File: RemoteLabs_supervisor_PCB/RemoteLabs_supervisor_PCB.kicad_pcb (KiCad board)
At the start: 4 copper layers, 180.3 x 99.1 mm, 200 parts, among them J1 Super_Prog_Header, J10 ShiftReg_Header, J11 SPI Student, J12 MCU_Header, J13 USB_B_Mini, J14 ShiftReg_Header, J15 SPI Supervisor, J16 MotorController_PWR_IP, J17 MotorController, J18 DC Motor Output, J19 Stepper Motor Output, J2 WS2821B Header, J20 Servo_A, J21 Servo_B, J22 Thermocouple A, J23 limit_switch_A, J24 limit_switch_B, J25 Optical Encoder, J26 Student_Prog_Header, J27 Analog Buffer, J28 student_PA03, J29 3V3 PWR SRC, J3 XT60_60A_male, J30 12V_DC, J31 5V_DC_RPI, J32 GND_BUS, J33 12V_BUS, J34 5V_P_BUS, J35 5V_D_BUS, J36 3V3_BUS, J4 Strip Lighting, J5 USB_A_Stacked, J6 5V_DC_LED, J7 USB_B_Mini, J8 MCU_Header, J9 Spare Student GPIOs, Q1 IRF5305_PBF, SW1 Stepper_Mode, SW2 Student Reset, SW3 Supervisor Reset, U1 R-78C5.0-1.0, U10 4081, U11 4081, U12 4081, U13 74HC86, U14 74HC86, U15 NCS20074D, U16 NCS20074D, U17 NCS20074D, U18 R-78C5.0-1.0, U19 AD8497, U2 TCYSH14F, U20 74LS07, U21 74LS07, U22 74LS07, U23 TCYSH14F, U3 AMS1117-3.3, U4 ATSAMD21G18A-M, U5 4094, U6 ATSAMD21G18A-M, U7 4094, U8 4069, U9 4081, X1 ASEK-xxxMHz, X2 ASEK-xxxMHz

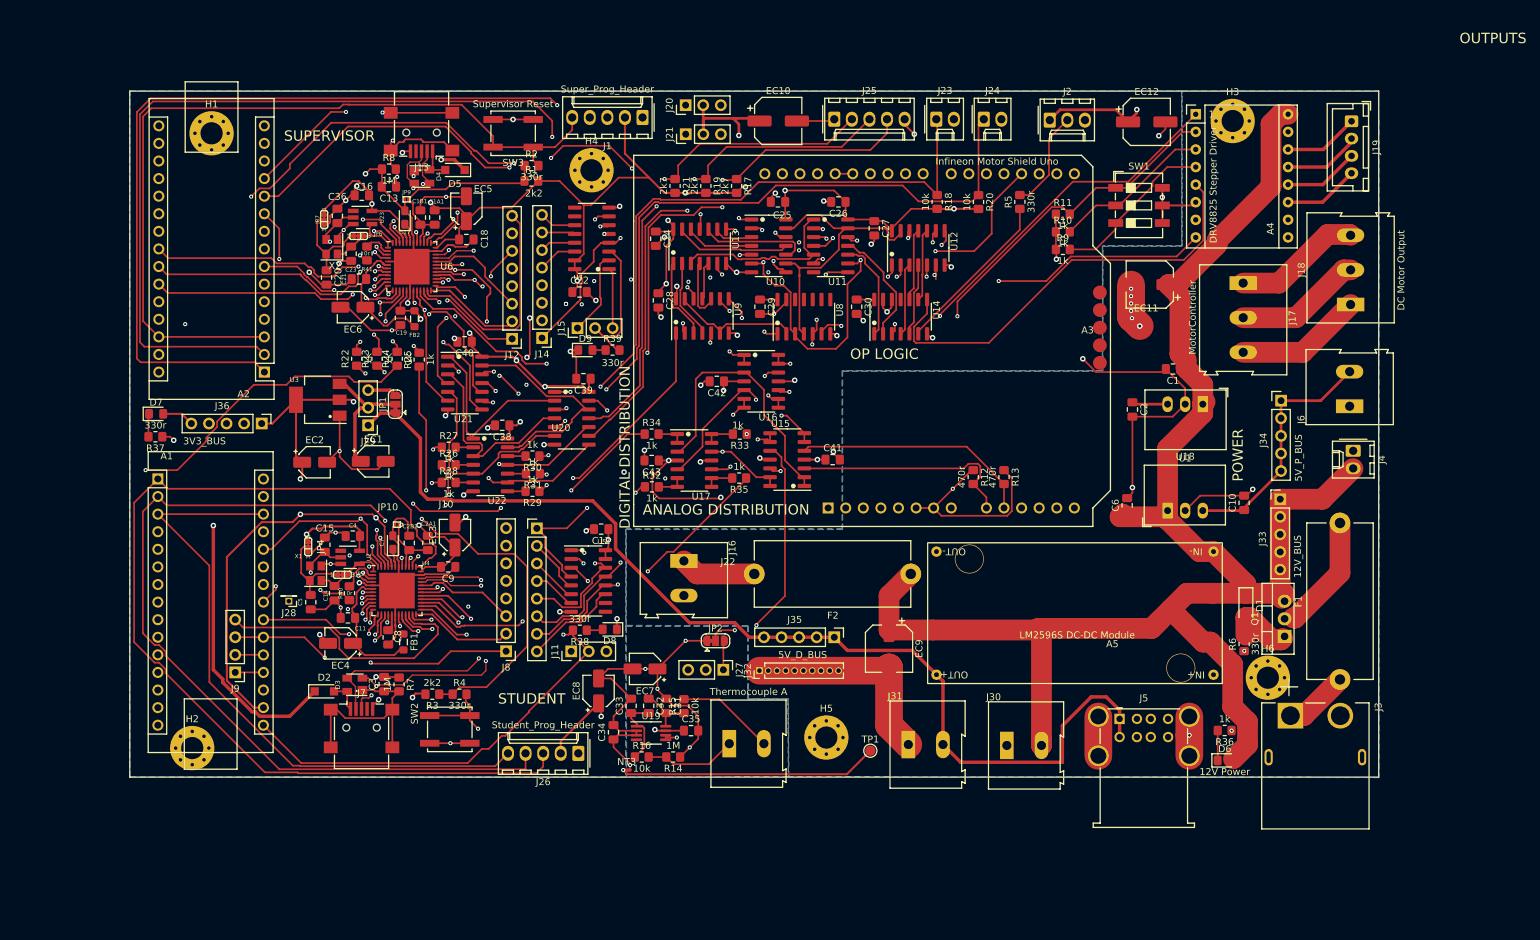
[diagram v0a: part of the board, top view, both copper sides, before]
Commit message: routing board layout 2.0
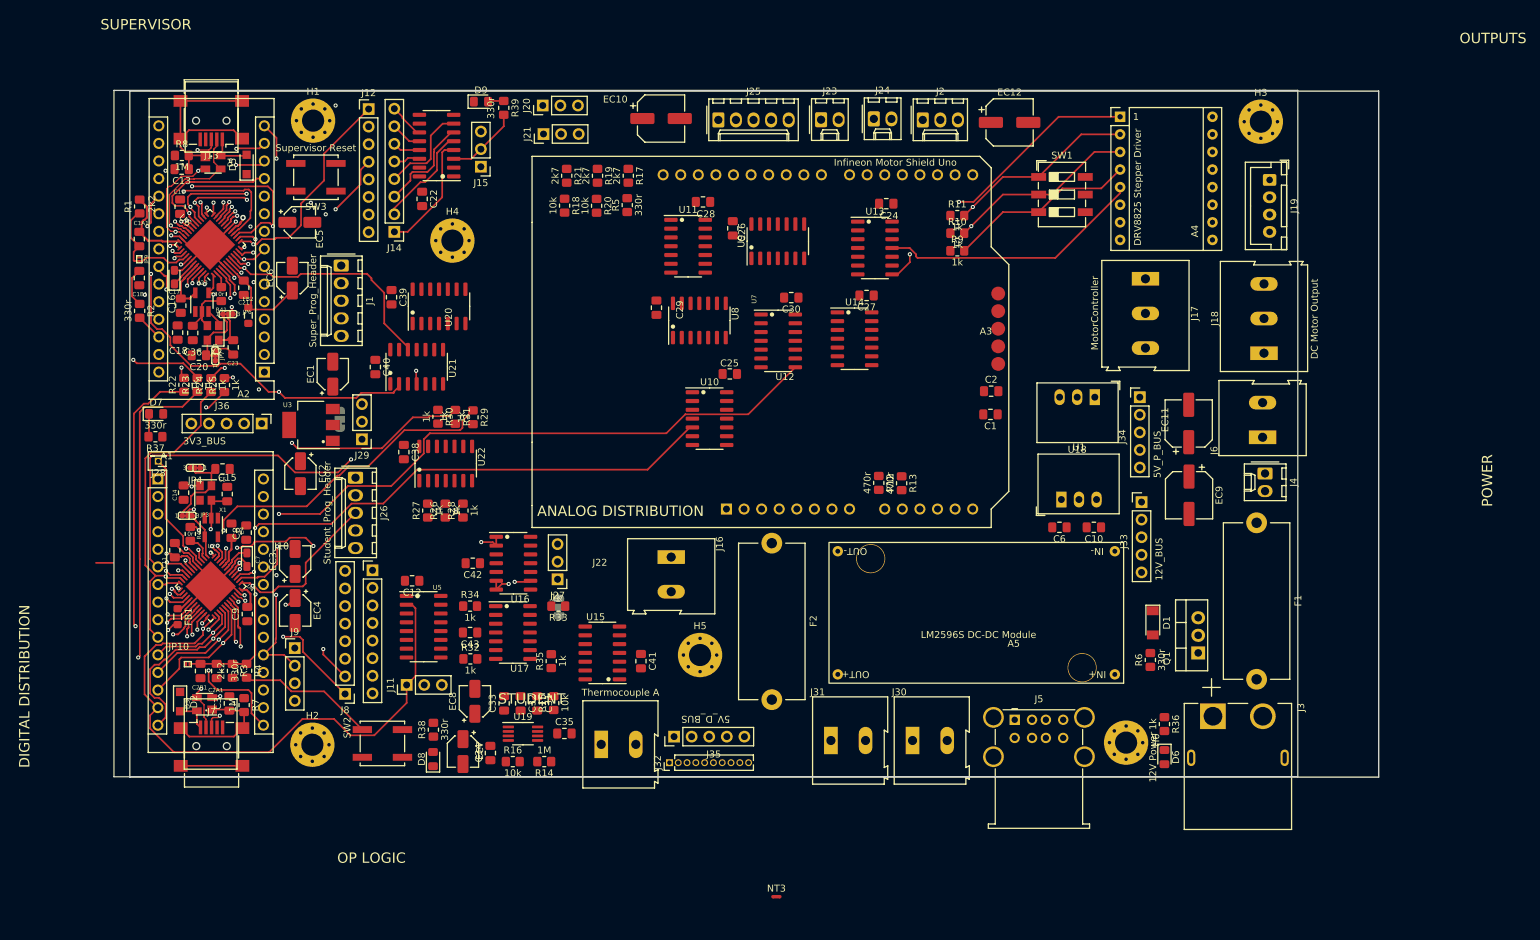
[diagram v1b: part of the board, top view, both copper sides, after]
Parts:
- removed TP1: GND, TestPoint:TestPoint_Pad_D1.5mm
- removed the U12 at (164.7, 45.5)
- added U9: 4081, Package_SO:SOIC-14_3.9x8.7mm_P1.27mm, F.Cu at (144.4, 44.5)
- JP1, JP2: moved to B.Cu
- moved R2 60.4 mm to (52.2, 54.6), turned to -90 degrees
- moved R5 56.7 mm to (122.6, 39.3)
- moved R1 56.7 mm to (52.2, 39.5), turned to 90 degrees
- moved R20 55.1 mm to (118.2, 39.4)
- moved R18 53.8 mm to (113.6, 39.4)
- moved J26 51.2 mm to (83.4, 78.7), turned to -90 degrees
- moved EC9 48.7 mm to (203.8, 81.2)
- moved J1 48.5 mm to (81.3, 48.1), turned to -90 degrees
- moved U16 44.4 mm to (106.2, 91.0)
- moved C42 43.9 mm to (100.3, 91.0)
- moved C18 43.8 mm to (57.7, 57.7), turned to -90 degrees
- moved C1A1 42.8 mm to (52.2, 44.2)
- moved C1B1 41.5 mm to (52.2, 49.9), turned to -90 degrees
- moved C41 40.2 mm to (124.6, 105.2), turned to -90 degrees
- moved JP9 39.6 mm to (52.2, 47.1), turned to -90 degrees
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- renumbered U9 to U12
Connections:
- U10 pad 12: /Output Logic/SUPERVISOR_STEP -> /Output Logic/STUDENT_STEP_RST
- U10 pad 13: Net-(U10-Pad13) -> /Output Logic/MCU_STEP_SELECT
- U10 pad 8: /Output Logic/SUPERVISOR_DIRECTION -> /Output Logic/STUDENT_STEP_EN
- U10 pad 9: Net-(U10-Pad13) -> /Output Logic/MCU_STEP_SELECT
- U11 pad 1: Net-(U11-Pad1) -> /Output Logic/SUPERVISOR_DIRECTION
- U11 pad 12: /Output Logic/SUPERVISOR_STEP_EN -> /Output Logic/SUPERVISOR_STEP_RST
- U11 pad 13: Net-(U10-Pad13) -> Net-(U11-Pad2)
- U11 pad 2: /Output Logic/MOTOR_DIR_A -> Net-(U11-Pad2)
- U11 pad 3: /DC Motor Controller/IN_1 -> Net-(U11-Pad3)
- U11 pad 4: /DC Motor Controller/IN_2 -> Net-(U11-Pad4)
- U11 pad 5: Net-(U11-Pad1) -> /Output Logic/SUPERVISOR_STEP
- U11 pad 6: /Output Logic/MOTOR_DIR_B -> Net-(U11-Pad2)
- U11 pad 8: /Output Logic/STUDENT_STEP_EN -> /Output Logic/SUPERVISOR_STEP_EN
- U11 pad 9: /Output Logic/MCU_STEP_SELECT -> Net-(U11-Pad2)
- U12 pad 10: Net-(U13-Pad4) -> Net-(U12-Pad10)
- U12 pad 11: Net-(U13-Pad5) -> Net-(U12-Pad11)
- U12 pad 12: /Output Logic/SUPERVISOR_MOTOR_EN -> /Output Logic/SUPERVISOR_PIXEL_DATA
- U12 pad 13: Net-(U8-Pad2) -> Net-(U12-Pad13)
- U12 pad 3: Net-(U13-Pad1) -> Net-(U14-Pad1)
- U12 pad 4: Net-(U13-Pad2) -> Net-(U14-Pad4)
- U12 pad 5: /Output Logic/SUPERVISOR_MOTOR_PWM -> /Output Logic/STUDENT_MOTOR_EN
- U12 pad 6: Net-(U8-Pad2) -> /Output Logic/MCU_MOTOR_SELECT
- U12 pad 8: /Output Logic/STUDENT_MOTOR_EN -> /Output Logic/STUDENT_PIXEL_DATA
- U12 pad 9: /Output Logic/MCU_MOTOR_SELECT -> /Output Logic/MCU_PIXEL_SELECT
- U13 pad 1: Net-(U13-Pad1) -> Net-(U10-Pad3)
- U13 pad 10: Net-(U10-Pad10) -> Net-(U11-Pad10)
- U13 pad 11: /Output Logic/STEPP_STEP_OUT -> /Output Logic/STEP_RST_OUT
- U13 pad 12: Net-(U10-Pad4) -> Net-(U10-Pad11)
- U13 pad 13: Net-(U10-Pad11) -> Net-(U11-Pad11)
- U13 pad 2: Net-(U13-Pad2) -> Net-(U11-Pad3)
- U13 pad 3: Net-(U11-Pad1) -> /Output Logic/DIRECTION_OUT
- U13 pad 4: Net-(U13-Pad4) -> Net-(U10-Pad4)
- U13 pad 5: Net-(U13-Pad5) -> Net-(U11-Pad4)
- U13 pad 6: /DC Motor Controller/ENABLE -> /Output Logic/STEPP_STEP_OUT
- U13 pad 8: /Output Logic/DIRECTION_OUT -> /Output Logic/STEP_EN_OUT
- U13 pad 9: Net-(U10-Pad3) -> Net-(U10-Pad10)
- U14 pad 1: Net-(U11-Pad10) -> Net-(U14-Pad1)
- U14 pad 2: Net-(U11-Pad11) -> Net-(U14-Pad2)
- U14 pad 3: /Output Logic/STEP_EN_OUT -> Net-(U9-Pad1)
- U14 pad 4: Net-(U12-Pad3) -> Net-(U14-Pad4)
- U14 pad 6: /Output Logic/PIXEL_DATA_OUT -> /DC Motor Controller/ENABLE
- U14 pad 8: /Output Logic/STEP_RST_OUT -> /Output Logic/PIXEL_DATA_OUT
- U8 pad 4: Net-(U10-Pad13) -> Net-(U11-Pad2)
- U8 pad 6: Net-(U12-Pad6) -> Net-(U12-Pad13)
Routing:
- net 3V3_DC_MCU: track 694.5 -> 33.7 mm, vias 34 -> 1
- net GNDD: track 417.2 -> 60.5 mm, vias 58 -> 5
- net 12V_DC_BUS: track 239.1 -> 0.00 mm
- net USB_BUS: track 163.2 -> 0.00 mm, vias 2 -> 0
- net 5V_DC_RPI: track 154.0 -> 0.00 mm
- net /Output Logic/MOTOR_DIR_B: track 148.0 -> 13.5 mm, vias 5 -> 1
- net 5V_DC_LED: track 118.0 -> 0.00 mm, vias 1 -> 0
- net STPPR_FAULT: track 116.3 -> 0.00 mm, vias 1 -> 0
- net /Supervisor MCU/PROG_TX: track 153.3 -> 43.0 mm, vias 2 -> 1
- net SERVO_1: track 130.2 -> 20.6 mm, vias 2 -> 1
- net /Output Logic/SUPERVISOR_PIXEL_DATA: track 112.9 -> 5.17 mm, vias 3 -> 1
- net /Output Logic/SUPERVISOR_STEP: track 116.9 -> 9.49 mm, vias 4 -> 1
- net /Supervisor MCU/PROG_RX: track 147.8 -> 42.0 mm, vias 2 -> 1
- net /Output Logic/STUDENT_STEP_RST: track 101.7 -> 0.00 mm, vias 2 -> 0
- net 5V_DC_SERVO: track 101.6 -> 0.00 mm, vias 1 -> 0
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- removed copper zone on B.Cu, net GNDA
- removed copper zone on B.Cu, net GNDD
- removed copper zone on B.Cu, net GNDPWR
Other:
- board size 180.3 x 99.1 mm -> 182.6 x 99.2 mm
